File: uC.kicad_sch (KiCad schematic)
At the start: 26 parts, among them J1 Conn_02x03_ESP_PROG, J12 UEXT_Host, J2 I2C Conn, J4 MCU head, J5 UART (CAN) Conn, P2 QTGM027, SW1 SW_Push, U2 ESP32-S3-WROOM-1-N4

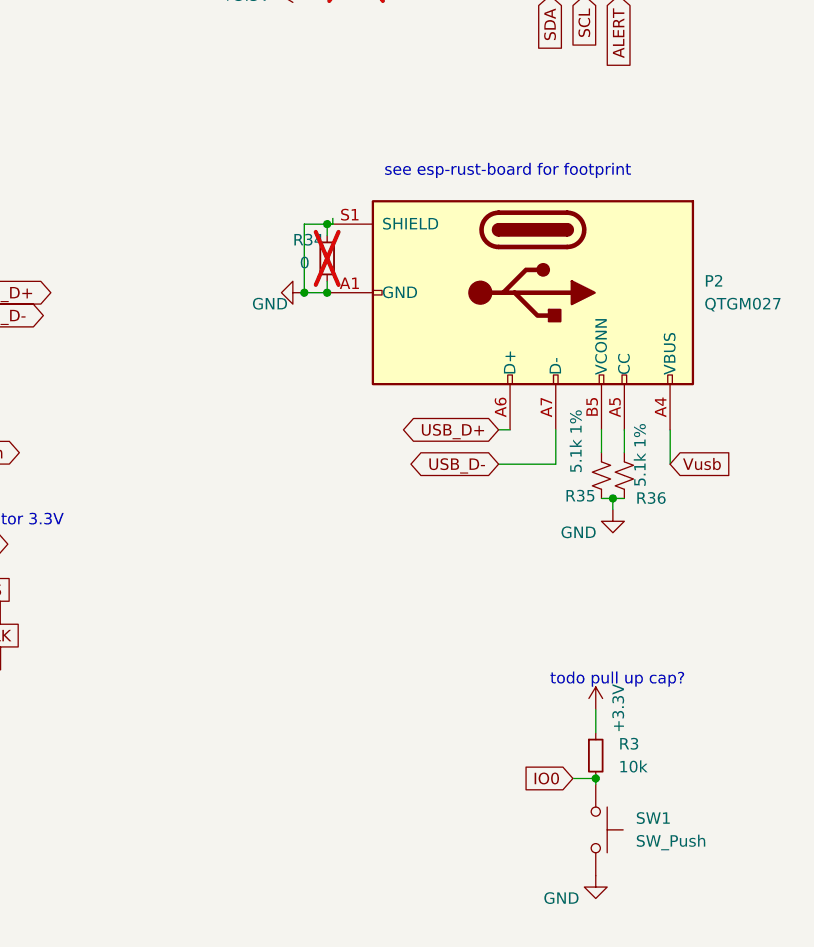
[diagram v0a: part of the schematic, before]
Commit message: Add RC connection between USB-C shield and GND
1. Added a 1 MΩ resistor and 10 nF capacitor between the USB Type-C connector shield and GND in the schematic and PCB layout.
2. Added clearer USB connector symbol having no missing pads
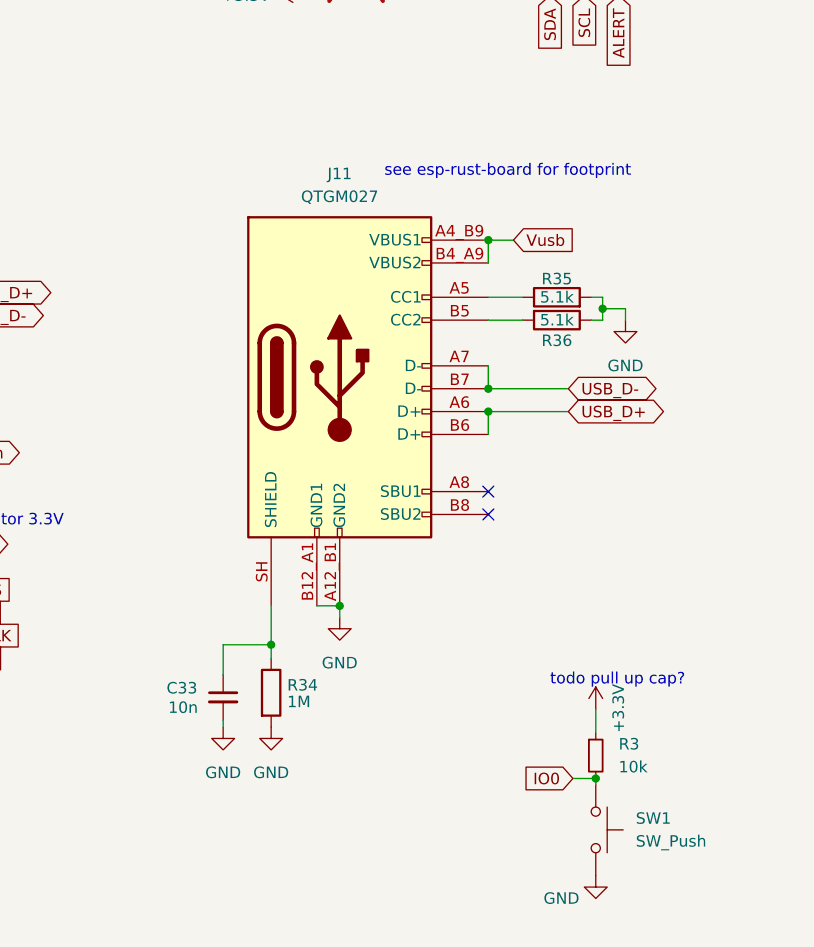
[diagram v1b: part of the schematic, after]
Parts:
- removed P2: QTGM027, open-pe:USB_C_Receptacle_GCT_USB4105-xx-A_16P_TopMnt_Horizontal, symbol Connector:USB_C_Plug_USB2.0
- removed R34: 0, Resistor_SMD:R_0402_1005Metric, symbol Device:R_Small
- removed R35, R36: 5.1k 1%, Resistor_SMD:R_0402_1005Metric, symbol Device:R_Small_US
- added C33: 10n, Capacitor_SMD:C_0402_1005Metric, symbol Device:C_Small
- added J11: QTGM027, UJ20-C-G-MSMT-TR-68:CUI_UJ20-C-G-MSMT-TR-68, symbol usb_c_receptacle_usb2.0_16p_8dummy:USB_C_Receptacle_USB2.0_16P
- added R34: 1M, Resistor_SMD:R_0402_1005Metric, symbol Device:R
- added R35, R36: 5.1k, Resistor_SMD:R_0402_1005Metric, symbol Device:R
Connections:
- net GND: now also C33.2, J11.A12_B1 (GND2), J11.B12_A1 (GND1), R34.2, R35.2, R36.1
- net USB_D+: now also J11.A6 (D+), J11.B6 (D+)
- net USB_D-: now also J11.A7 (D-), J11.B7 (D-)
- net Vusb: now also J11.A4_B9 (VBUS1), J11.B4_A9 (VBUS2)
- new net: J11.A5 (CC1), R35.1
- new net: C33.1, J11.SH (SHIELD), R34.1
- new net: J11.B5 (CC2), R36.2
- no-connect marks 14 -> 16
